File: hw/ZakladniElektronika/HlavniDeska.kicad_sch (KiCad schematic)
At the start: 0 parts

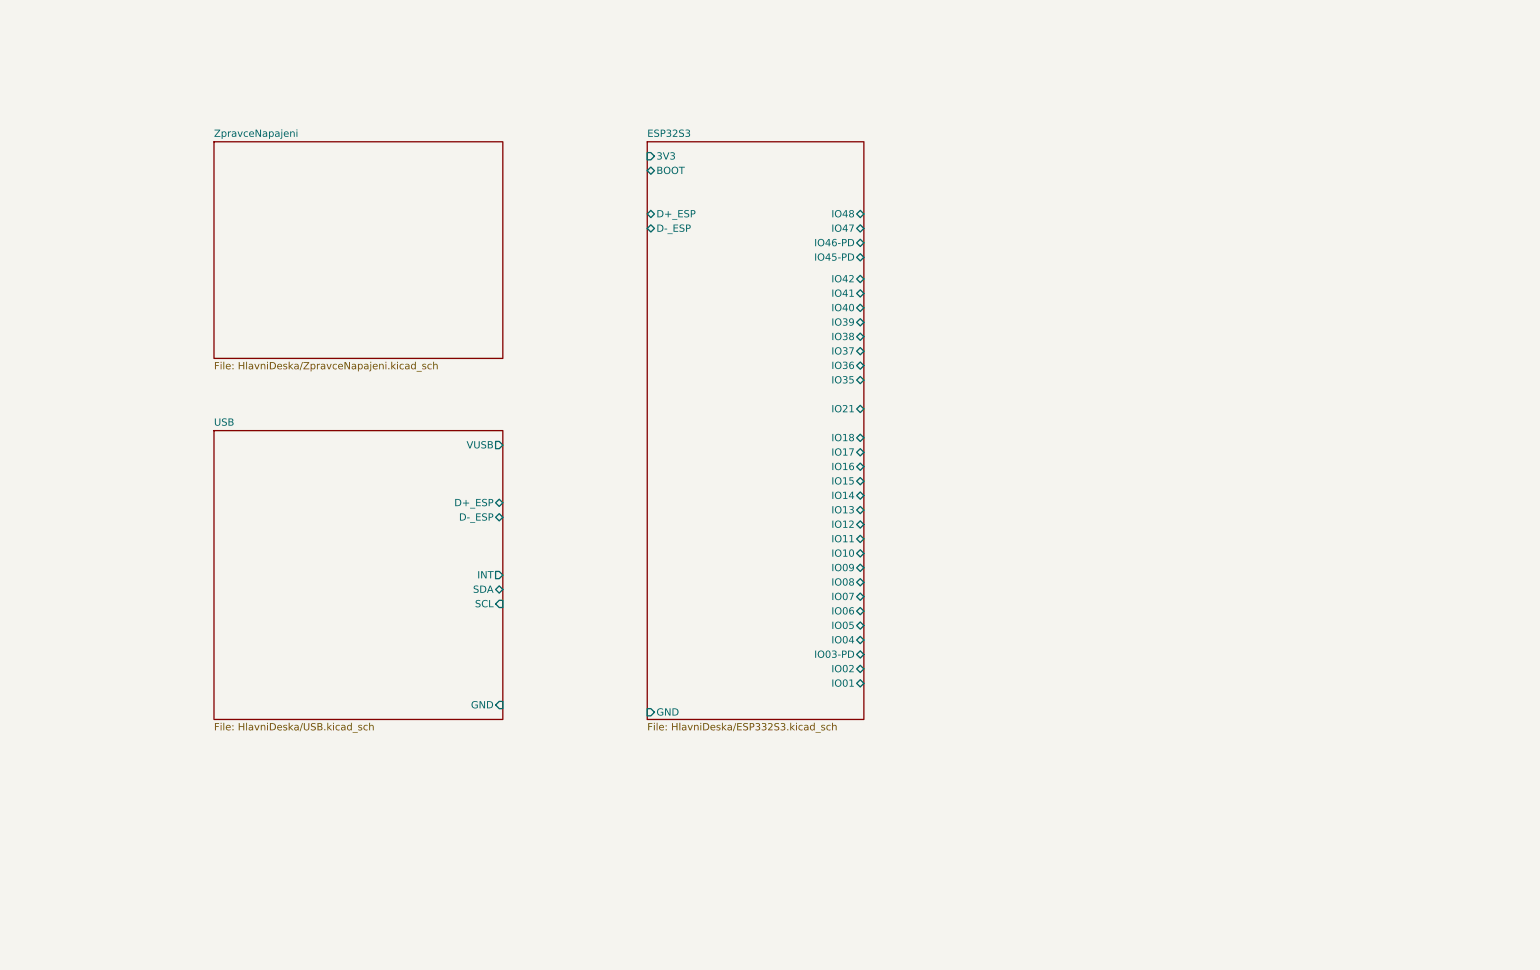
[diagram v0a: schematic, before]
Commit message: WIP
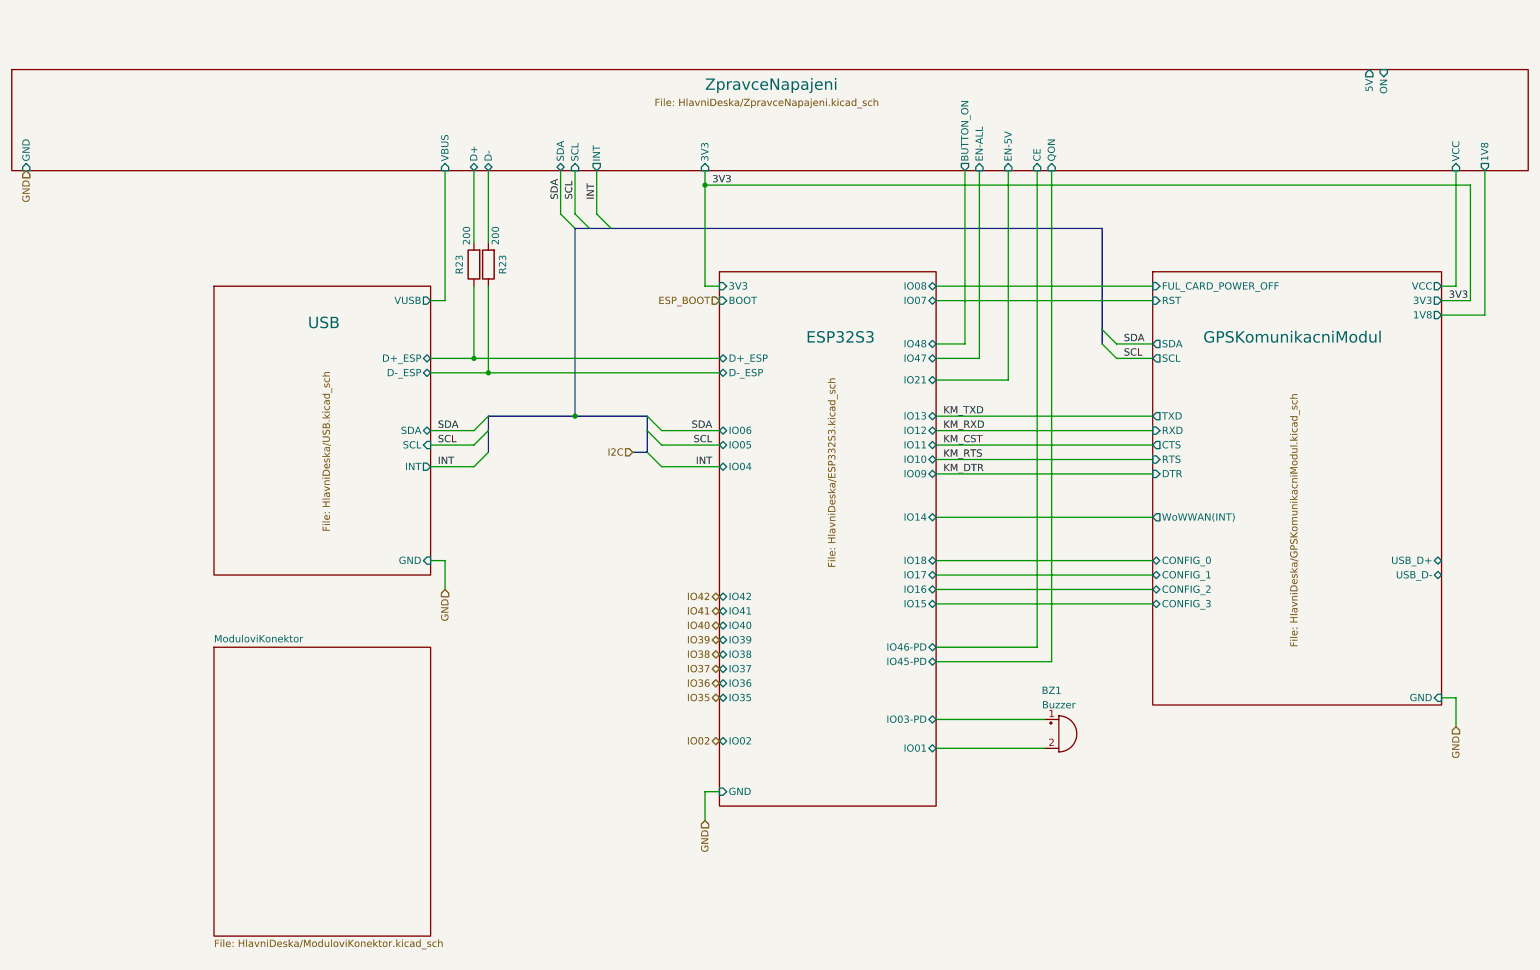
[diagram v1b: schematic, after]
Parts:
- added BZ1: Buzzer, Robotarna_KiCad_Library:PKLCS1212E-(RH-Logic_piezzo), symbol Device:Buzzer
- added R23 (x2): 200, Resistor_SMD:R_0402_1005Metric, symbol Device:R
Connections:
- net ESP32S3/D+_ESP: now also R23.1
- net ESP32S3/D-_ESP: now also R23.1
- net ESP32S3/IO01: now also BZ1.2 (+)
- net ESP32S3/IO03-PD: now also BZ1.1 (-)
- new net ZpravceNapajeni/D+: R23.2
- new net ZpravceNapajeni/D-: R23.2
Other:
- added sheet GPSKomunikacniModul (HlavniDeska/GPSKomunikacniModul.kicad_sch)
- added sheet ModuloviKonektor (HlavniDeska/ModuloviKonektor.kicad_sch)
- sheet ZpravceNapajeni ports: added 1V8, 3V3, 5V, BUTTON_ON, CE, D+, D-, EN-5V, EN-ALL, GND, INT, ON, QON, SCL, SDA, VBUS, VCC; removed none

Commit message: Nastin schematu
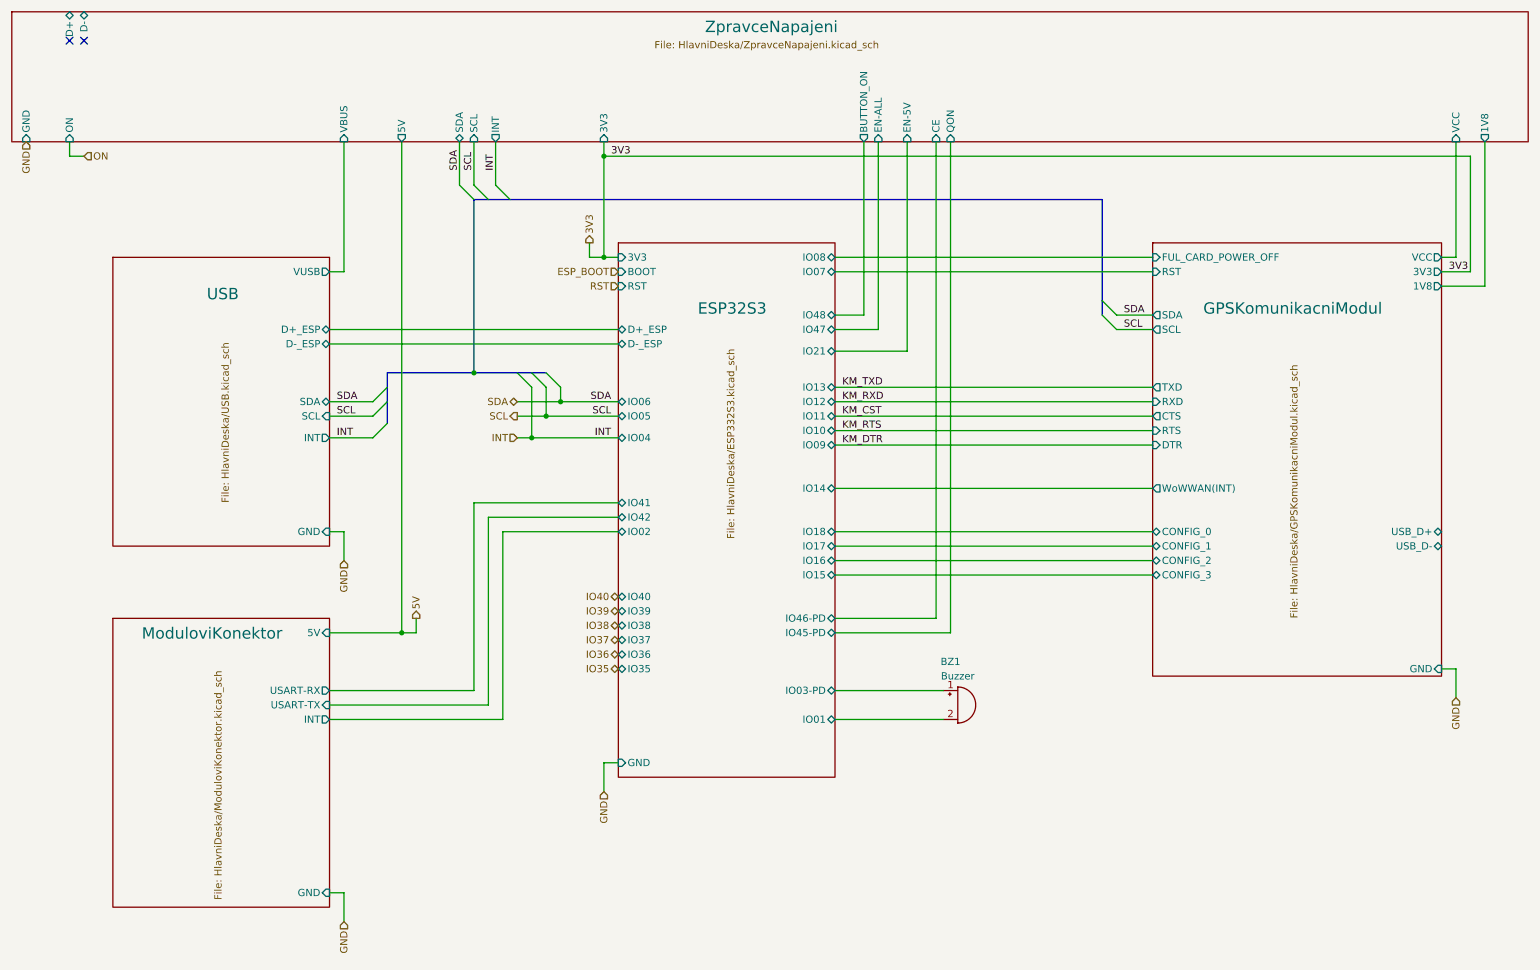
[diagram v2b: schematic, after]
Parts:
- removed R23 (x2): 200, Resistor_SMD:R_0402_1005Metric, symbol Device:R
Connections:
- no-connect marks 0 -> 2
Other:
- sheet ESP32S3 ports: added RST; removed none
- sheet ModuloviKonektor ports: added 5V, GND, INT, USART-RX, USART-TX; removed none
- moved on the sheet: BZ1
